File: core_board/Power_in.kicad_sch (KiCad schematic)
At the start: 37 parts, among them J1 Molex_Megafit_02, Q1 TPC8132_LQS, U1 AP63301WU7, U2 AP63205QWU7, U4 AOZ6605PI-1

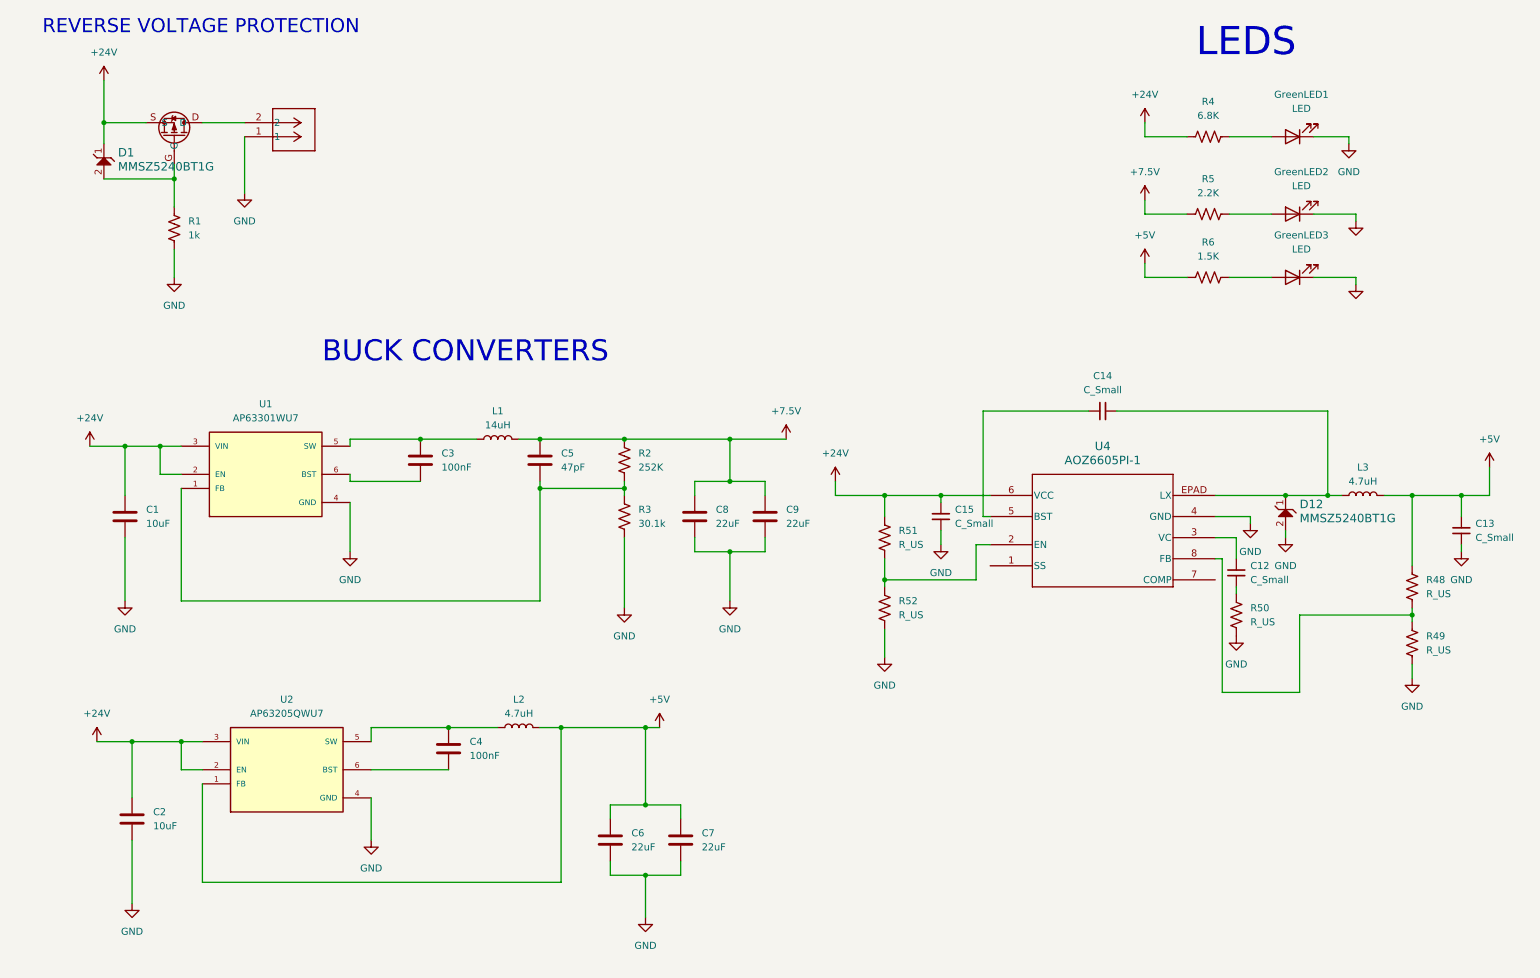
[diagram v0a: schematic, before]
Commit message: Almost done with Schematic
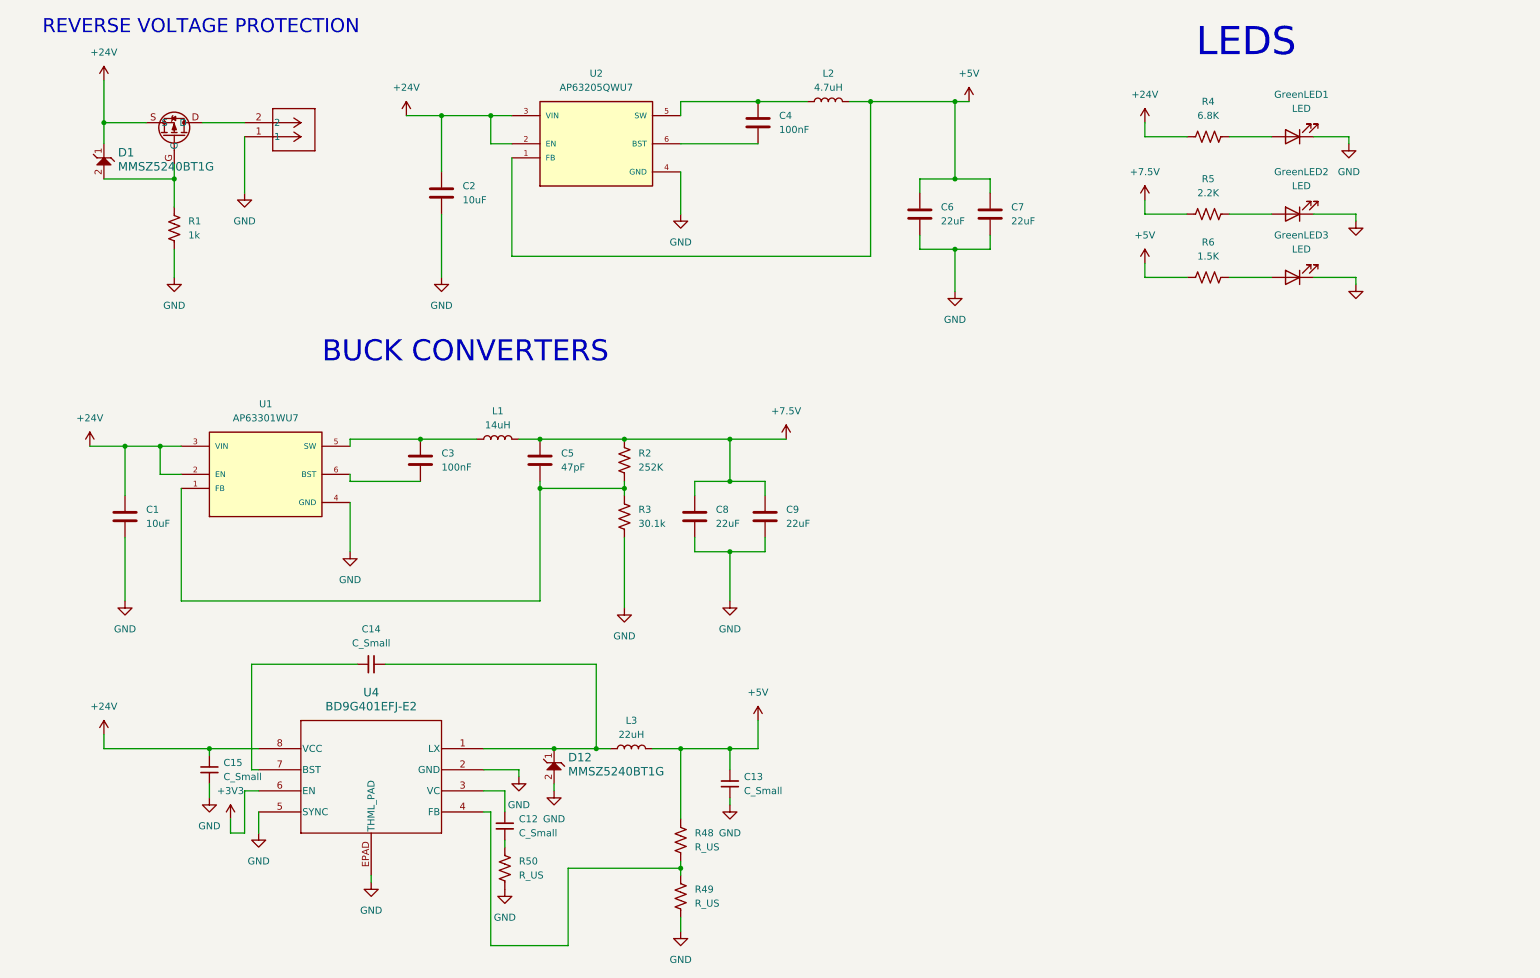
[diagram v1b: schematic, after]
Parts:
- removed R51, R52: R_US, Package_DFN_QFN:WDFN-10-1EP_3x3mm_P0.5mm_EP1.8x2.5mm, symbol Device:R_US
- C1, C12, C13, C14, C15, C2, C3, C4, C5, C6, C7, C8, C9: footprint Package_SO:SOIC-8_3.9x4.9mm_P1.27mm -> Capacitor_SMD:C_0603_1608Metric_Pad1.08x0.95mm_HandSolder
- D1, D12: footprint MRDT_Devices:SOD-123_ONS-L -> LED_SMD:LED_0603_1608Metric_Pad1.05x0.95mm_HandSolder
- GreenLED1: footprint Inductor_SMD:L_0603_1608Metric_Pad1.05x0.95mm_HandSolder -> LED_SMD:LED_0603_1608Metric_Pad1.05x0.95mm_HandSolder
- L1, L2: footprint OptoDevice:Everlight_ITR9608-F -> (none)
- L3: value 4.7uH -> 22uH; footprint OptoDevice:Everlight_ITR9608-F -> AMRM00101040220MA1:IND_AMRM00101040_PUL
- R1, R2, R3, R4, R5, R6: footprint Package_DIP:DIP-8_W7.62mm -> Resistor_SMD:R_0603_1608Metric_Pad0.98x0.95mm_HandSolder
- R48, R50: footprint Package_DFN_QFN:WDFN-10-1EP_3x3mm_P0.5mm_EP1.8x2.5mm -> Resistor_SMD:R_0603_1608Metric_Pad0.98x0.95mm_HandSolder
- R49: footprint (none) -> Resistor_SMD:R_0603_1608Metric_Pad0.98x0.95mm_HandSolder
- U1, U2: footprint AP63205QWU7:SOT95P280X100-6N -> Package_TO_SOT_SMD:SOT-23-6_Handsoldering
- U4: value AOZ6605PI-1 -> BD9G401EFJ-E2; footprint SOIC-8:SO8_EP1_AOS -> Package_SO:SOIC-8-1EP_3.9x4.9mm_P1.27mm_EP2.29x3mm
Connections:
- net +24V: now also U4.8 (VCC); no longer U4.6 (VCC)
- net GND: now also U4.2 (GND), U4.5 (SYNC), U4.EPAD (THML_PAD); no longer U4.4 (GND)
- net at C14.1: now also U4.7 (BST); no longer U4.5 (BST)
- net at C14.2, D12.1, L3.1: now also U4.1 (LX); no longer U4.EPAD (LX)
- net at R48.2, R49.1: now also U4.4 (FB); no longer U4.8 (FB)
- new net +3V3: U4.6 (EN)
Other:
- moved on the sheet: C12, C13, C14, C15, C2, C4, C6, C7, D12, L2, L3, R48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

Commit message: add
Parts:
- L1: footprint (none) -> Inductor_SMD:L_TechFuse_SL1050
- L2: footprint (none) -> Inductor_SMD:L_0603_1608Metric
